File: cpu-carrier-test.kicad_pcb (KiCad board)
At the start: 4 copper layers, 151.6 x 172.3 mm, 191 parts, among them J1 Micro_SD_Card_Det, J1101 USB_miniB, J1102 USB_C_Receptacle_USB2.0, J19 SFP, J20 SFP_CAGE, J2001 BNC, J2051 BNC, J2201 BEL_0845_2G1T_H5, J4 JTAG, J5 Molex_0936263508, J6 USB_A, SW1 SW_Push, SW2101 SW_DIP_x08, U1 TXS0108EPW, U1101 USB3740B-AI9, U1102 UTC2000, U1103 FT232RL, U1104 74LVC1G00, U1105 SC185, U2001 74LVC2T45DC, U2051 74LVC2T45DC, U2101 74LVC1G06, U2102 74LVC1G06, U2103 PCA9306, U2104 24AA0x, U2201 74LVC1G06, U2202 74LVC1G06, U2301 lan9254, U6 PCA9546AD, U8 74AC125, U9 TPS2051B, X2301 FNETHE025

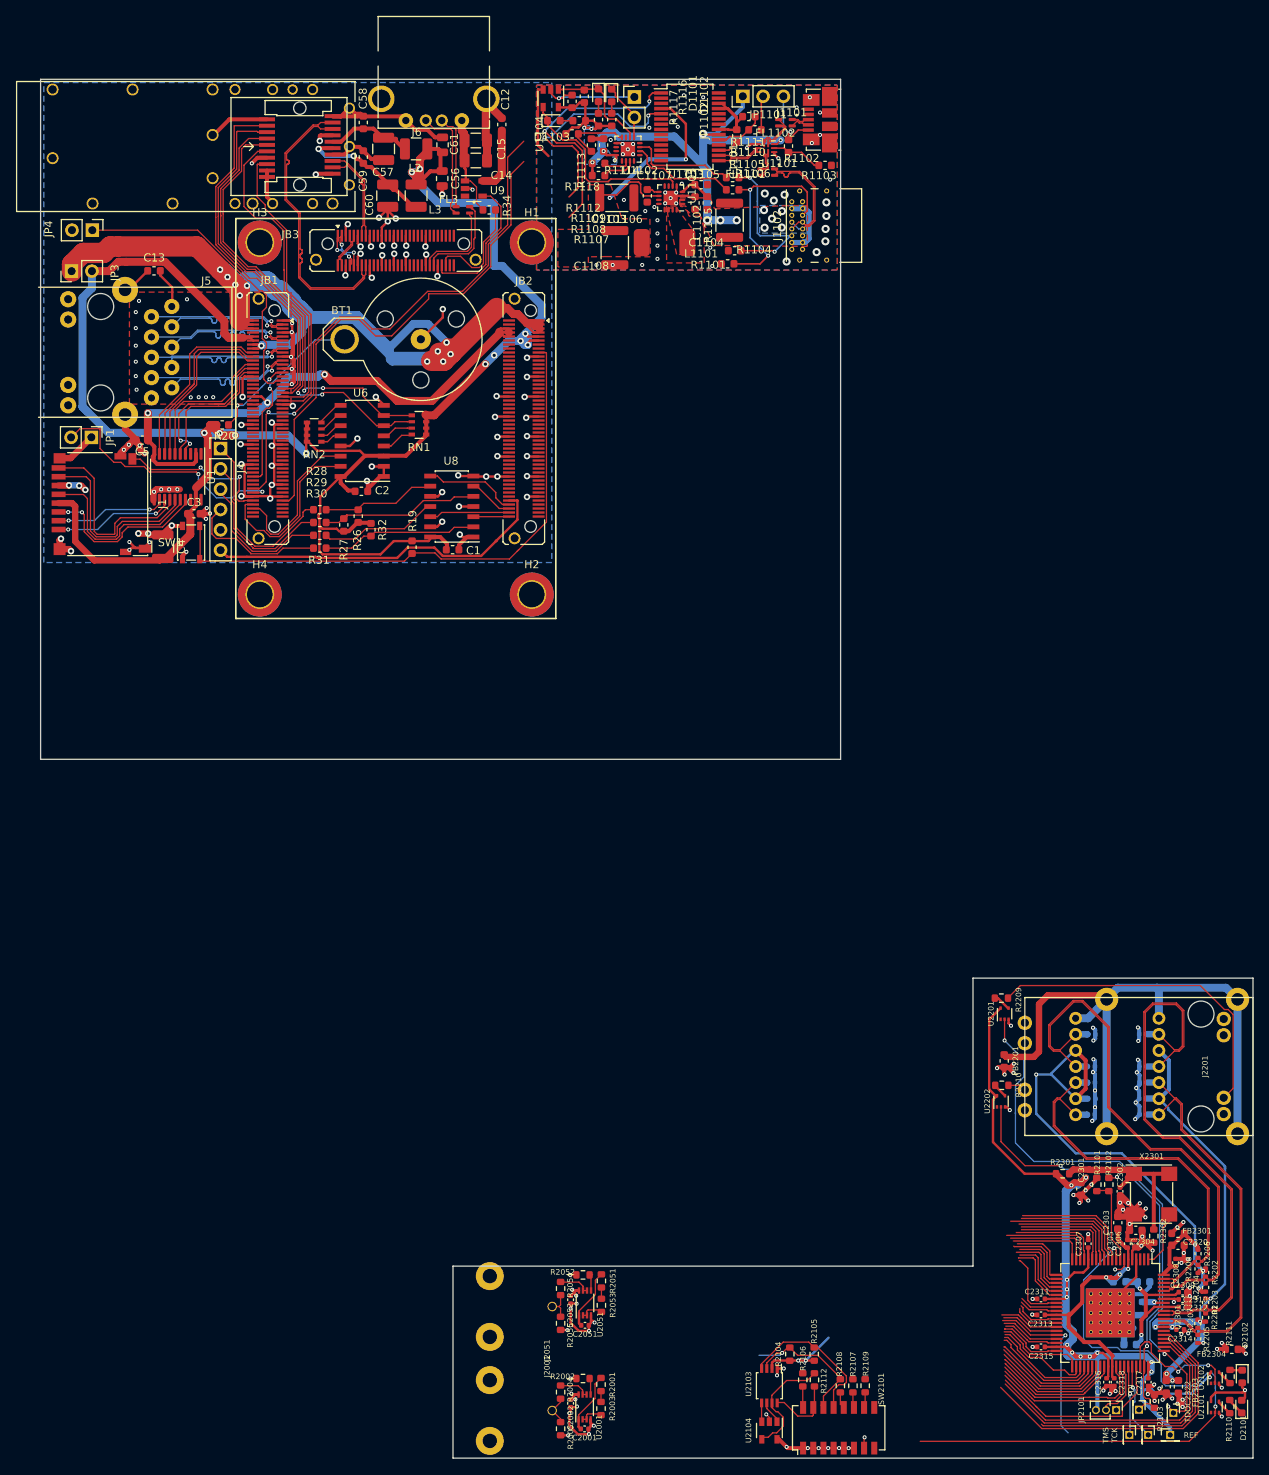
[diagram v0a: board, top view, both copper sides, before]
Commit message: cont. work; all connections done now
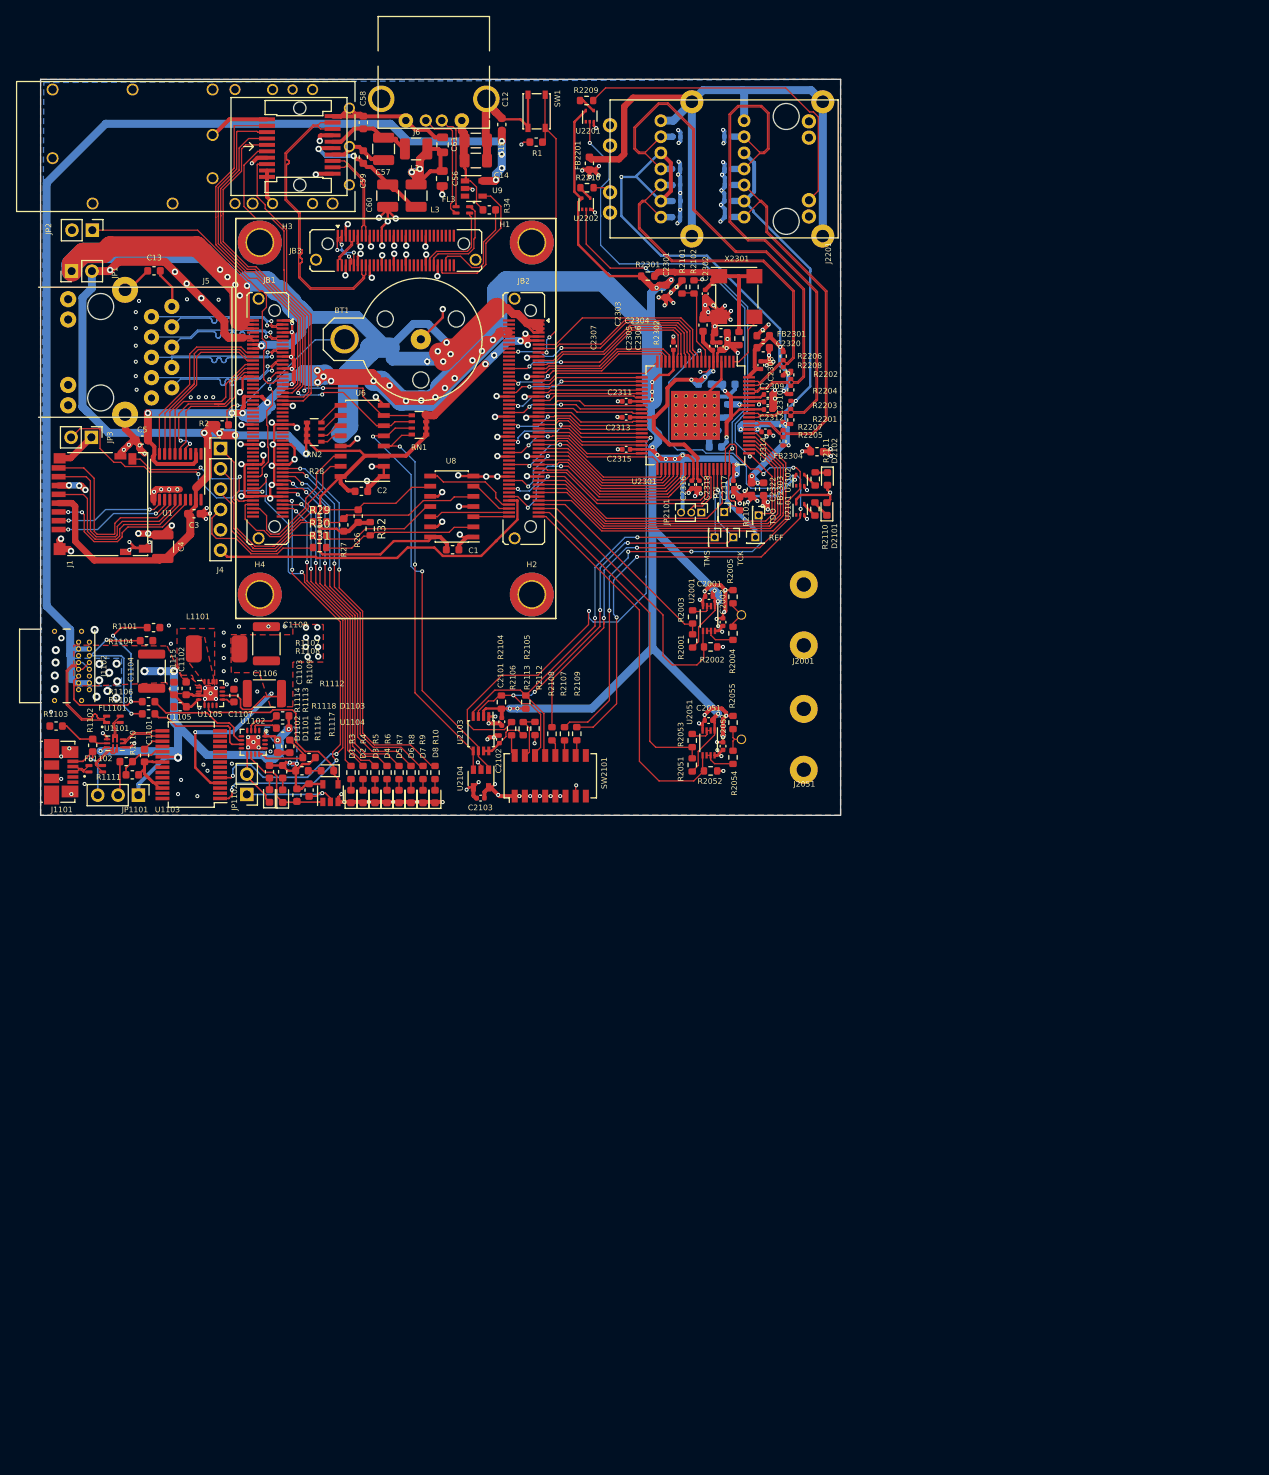
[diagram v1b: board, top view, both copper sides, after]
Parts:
- added C2101: 100n, Capacitor_SMD:C_0402_1005Metric, F.Cu at (157.7, 110.3)
- added C2102: 100p, Capacitor_SMD:C_0402_1005Metric, F.Cu at (157.3, 112.5)
- added C2103: 100n, Capacitor_SMD:C_0402_1005Metric, F.Cu at (155.0, 119.8)
- added D1: LED, LED_SMD:LED_0603_1608Metric, F.Cu at (138.8, 119.7)
- added D2: LED, LED_SMD:LED_0603_1608Metric, F.Cu at (140.3, 119.7)
- added D3: LED, LED_SMD:LED_0603_1608Metric, F.Cu at (141.8, 119.7)
- added D4: LED, LED_SMD:LED_0603_1608Metric, F.Cu at (143.3, 119.7)
- added D5: LED, LED_SMD:LED_0603_1608Metric, F.Cu at (144.8, 119.7)
- added D6: LED, LED_SMD:LED_0603_1608Metric, F.Cu at (146.3, 119.7)
- added D7: LED, LED_SMD:LED_0603_1608Metric, F.Cu at (147.8, 119.7)
- added D8: LED, LED_SMD:LED_0603_1608Metric, F.Cu at (149.3, 119.7)
- added R10: 1k, Resistor_SMD:R_0603_1608Metric, F.Cu at (149.3, 116.7)
- added R2113: 100k, Resistor_SMD:R_0603_1608Metric, F.Cu at (161.8, 111.2)
- added R3: 1k, Resistor_SMD:R_0603_1608Metric, F.Cu at (138.8, 116.7)
- added R4: 1k, Resistor_SMD:R_0603_1608Metric, F.Cu at (140.3, 116.7)
- added R5: 1k, Resistor_SMD:R_0603_1608Metric, F.Cu at (141.8, 116.7)
- added R6: 1k, Resistor_SMD:R_0603_1608Metric, F.Cu at (143.3, 116.7)
- added R7: 1k, Resistor_SMD:R_0603_1608Metric, F.Cu at (144.8, 116.7)
- added R8: 1k, Resistor_SMD:R_0603_1608Metric, F.Cu at (146.3, 116.7)
- added R9: 1k, Resistor_SMD:R_0603_1608Metric, F.Cu at (147.8, 116.7)
- D2101, D2102: value LED_Small -> LED
- R1: renamed from R19; value R10k -> 10k
- R1102, R1103, R1116, R1117, R26, R27, R32: value R100k -> 100k
- R1105, R1106, R1107, R1108, R1111: value R10k -> 10k
- R1110: value R4k7 -> 5k1
- R2: renamed from R20; value R10k -> 10k
- R2104, R2105: value 10k -> 3k3
- R2109: value 4k7 -> 5k1
- R2112: value 10k -> 100k
- R28, R29, R30, R31: value R100 -> 100
- moved J1101 125.1 mm to (102.6, 116.6), turned to 270 degrees
- moved R2206 123.6 mm to (192.8, 64.6)
- moved TP2302 123.6 mm to (185.4, 84.1)
- moved U2102 123.6 mm to (194.9, 80.1)
- moved C2209 123.6 mm to (185.9, 45.2)
- moved C2302 123.6 mm to (183.1, 56.8)
- moved C2320 123.6 mm to (190.3, 63.5)
- moved FB2301 123.6 mm to (190.3, 62.0)
- moved J2201 123.6 mm to (193.2, 41.2)
- moved R2111 123.6 mm to (196.8, 80.0)
- moved U2202 123.6 mm to (168.2, 45.5)
- moved C2201 123.6 mm to (185.9, 37.1)
- moved C2303 123.6 mm to (182.8, 60.7)
- moved C2305 123.6 mm to (184.0, 63.4)
- moved C2306 123.6 mm to (184.9, 63.4)
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- renumbered JP3 to JP1, JP4 to JP2, JP1 to JP3
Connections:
- JB1 pad 75: /B2B Connector/B13_L18_P -> B13_L18_P
- JB1 pad 77: /B2B Connector/B13_L18_N -> B13_L18_N
- JB1 pad 79: /B2B Connector/B13_L21_N -> B13_L21_N
- JB1 pad 81: /B2B Connector/B13_L21_P -> B13_L21_P
- R2001 pad 2: /lan9254/FPGA_IO1_DAT -> B35_L10_P
- R2002 pad 1: /lan9254/FPGA_IO1_DIR -> B35_L20_N
- R2003 pad 1: /lan9254/FPGA_IO1_DAT -> B35_L10_P
- R2051 pad 2: /lan9254/FPGA_IO2_DAT -> B35_L20_P
- R2052 pad 1: /lan9254/FPGA_IO2_DIR -> B35_L25
- R2053 pad 1: /lan9254/FPGA_IO2_DAT -> B35_L20_P
- R2106 pad 1: /lan9254/FPGA_23 -> B35_L3_N
- R2108 pad 1: /lan9254/EESCL -> /lan9254/RUNLED
- R2112 pad 1: +3V3 -> Net-(R2112-Pad1)
- R2112 pad 2: Net-(R2112-Pad2) -> Net-(C2102-Pad1)
- SW2101 pad 15: Net-(R2112-Pad2) -> Net-(R2112-Pad1)
- U2001 pad 5: /lan9254/FPGA_IO1_DIR -> B35_L20_N
- U2051 pad 5: /lan9254/FPGA_IO2_DIR -> B35_L25
- U2102 pad 2: /lan9254/EESCL -> /lan9254/RUNLED
- U2103 pad 7: +3V3 -> Net-(C2102-Pad1)
- U2103 pad 8: Net-(R2112-Pad2) -> Net-(C2102-Pad1)
- U2301 pad 10: /lan9254/FPGA_0 -> B34_L15_N
- U2301 pad 11: /lan9254/FPGA_1 -> B34_L15_P
- U2301 pad 12: /lan9254/FPGA_2 -> B34_L18_N
- U2301 pad 13: /lan9254/FPGA_3 -> B34_L2_P
- U2301 pad 14: /lan9254/FPGA_4 -> B34_L2_N
- U2301 pad 15: /lan9254/FPGA_5 -> B34_L12_P
- U2301 pad 17: /lan9254/FPGA_6 -> B34_L6_N
- U2301 pad 18: /lan9254/FPGA_7 -> B34_L6_P
- U2301 pad 19: /lan9254/FPGA_8 -> B34_L8_P
- U2301 pad 20: /lan9254/FPGA_9 -> B35_L16_P
- U2301 pad 21: /lan9254/FPGA_10 -> B35_L16_N
- U2301 pad 22: /lan9254/FPGA_11 -> B34_L7_N
- U2301 pad 23: /lan9254/FPGA_12 -> B35_L18_N
- U2301 pad 24: /lan9254/FPGA_13 -> B35_L18_P
- U2301 pad 25: /lan9254/FPGA_14 -> B35_L21_P
- U2301 pad 26: /lan9254/FPGA_15 -> B35_L15_N
- U2301 pad 28: /lan9254/FPGA_16 -> B35_L15_P
- U2301 pad 29: /lan9254/FPGA_17 -> B35_L8_P
- U2301 pad 30: /lan9254/FPGA_18 -> B35_L13_P
- U2301 pad 32: /lan9254/FPGA_19 -> B35_L13_N
- U2301 pad 33: /lan9254/FPGA_20 -> B35_L11_N
- U2301 pad 34: /lan9254/FPGA_21 -> B35_L14_P
- U2301 pad 35: /lan9254/FPGA_22 -> B35_L14_N
- U2301 pad 36: /lan9254/FPGA_23 -> B35_L3_N
- U2301 pad 37: /lan9254/FPGA_24 -> B35_L12_P
- U2301 pad 38: /lan9254/FPGA_25 -> B35_L12_N
- U2301 pad 40: /lan9254/FPGA_26 -> B35_L7_N
- U2301 pad 41: /lan9254/FPGA_27 -> B35_L23_N
- U2301 pad 42: /lan9254/FPGA_28 -> B35_L23_P
- U2301 pad 43: /lan9254/FPGA_29 -> B35_L4_P
- U2301 pad 44: /lan9254/FPGA_30 -> B35_L2_N
- U2301 pad 45: /lan9254/FPGA_31 -> B35_L2_P
- U2301 pad 46: /lan9254/FPGA_32 -> B35_L5_N
- U2301 pad 47: /lan9254/FPGA_33 -> B35_L17_P
- U2301 pad 48: /lan9254/FPGA_34 -> B35_L17_N
- U2301 pad 49: /lan9254/FPGA_35 -> B35_L6_N
- U2301 pad 52: /lan9254/FPGA_36 -> B35_L24_P
- U2301 pad 53: /lan9254/FPGA_37 -> B35_L24_N
- U2301 pad 57: /lan9254/FPGA_38 -> B35_L0
- U2301 pad 58: /lan9254/EESCL -> /lan9254/RUNLED
- U2301 pad 62: /lan9254/FPGA_39 -> B35_L9_N
- U2301 pad 63: /lan9254/FPGA_40 -> B35_L9_P
- U2301 pad 64: /lan9254/FPGA_41 -> B35_L22_N
- U2301 pad 65: /lan9254/FPGA_42 -> B35_L22_P
- U2301 pad 66: /lan9254/FPGA_43 -> B35_L10_N
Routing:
- net +1V8: track 221.3 -> 411.2 mm, vias 18 -> 36
- net +3V3_PWR_OUT: track 188.3 -> 329.7 mm, vias 13 -> 21
- net +5V: track 91.1 -> 218.3 mm, vias 15 -> 19
- net B35_L3_N: track 0.00 -> 79.0 mm, vias 0 -> 4
- net /lan9254/RUNLED: track 0.00 -> 69.9 mm, vias 0 -> 4
- net B13_L18_P: track 0.00 -> 49.6 mm, vias 0 -> 2
- net B35_L25: track 0.00 -> 48.1 mm
- net B13_L18_N: track 0.00 -> 47.8 mm, vias 0 -> 2
- net /lan9254/LINKACT0: track 70.7 -> 117.0 mm, vias 3 -> 5
- net B35_L10_N: track 0.00 -> 46.2 mm
- net SCL0: track 6.81 -> 52.9 mm, vias 0 -> 2
- net B13_L21_N: track 0.00 -> 46.0 mm, vias 0 -> 2
- net B35_L22_P: track 0.00 -> 45.3 mm
- net B13_L21_P: track 0.00 -> 44.6 mm, vias 0 -> 2
- net SDA0: track 6.38 -> 50.5 mm, vias 0 -> 2
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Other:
- board size 151.6 x 172.3 mm -> 100 x 92 mm
- net class diffp_ec: via_dia 0.4 -> 0.46
